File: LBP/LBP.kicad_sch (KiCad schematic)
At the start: 29 parts, among them U1 OPA1641, U2 OPA1641, U3 OPA1641, U4 OPA1641, U5 OPA1641

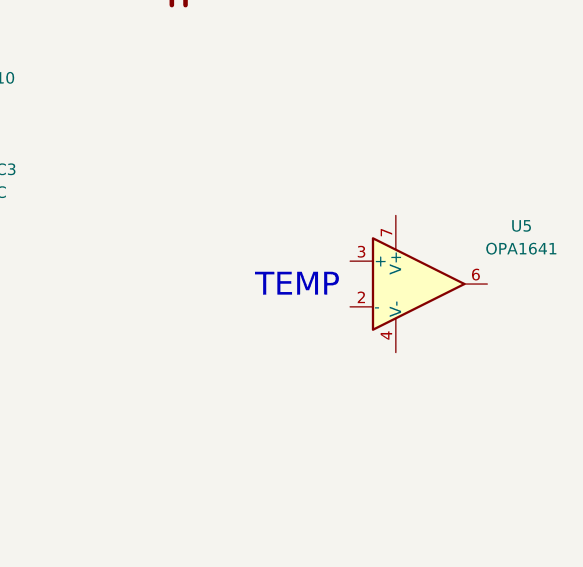
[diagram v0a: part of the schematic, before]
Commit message: LTspice jazz
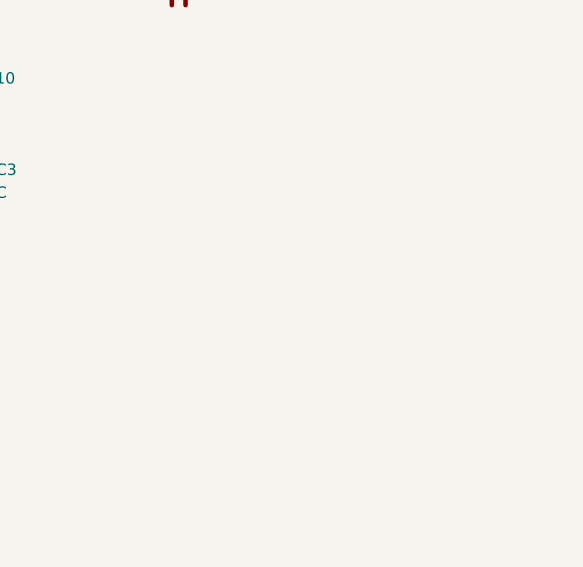
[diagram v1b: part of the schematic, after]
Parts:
- removed U5: OPA1641, symbol Amplifier_Operational:OPA1641
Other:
- note removed: "TEMP"
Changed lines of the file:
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@@
 		(rev "1.0")
-	)
-	(text "TEMP"
-		(exclude_from_sim no)
-		(at 151.638 81.534 0)
-		(effects
-			(font
-				(size 2.54 2.54)
-			)
-		)
 	)
 	(junction
@@
 					(unit 1)
 				)
-			)
-		)
-	)
-	(symbol
-		(lib_id "Amplifier_Operational:OPA1641")
-		(at 165.1 81.28 0)
-		(unit 1)
-		(exclude_from_sim no)
-		(in_bom yes)
-		(on_board yes)
-		(dnp no)
-		(fields_autoplaced yes)
-		(property "Reference" "U5"
-			(at 176.53 74.8598 0)
-			(effects
-				(font
-					(size 1.27 1.27)
-				)
-			)
-		)
-		(property "Value" "OPA1641"
-			(at 176.53 77.3998 0)
-			(effects
-				(font
-					(size 1.27 1.27)
-				)
-			)
-		)
-		(property "Footprint" ""
-			(at 165.1 81.28 0)
-			(effects
-				(font
-					(size 1.27 1.27)
-				)
-				(hide yes)
-			)
-		)
-		(property "Datasheet" "http://www.ti.com/lit/ds/symlink/opa1641.pdf"
-			(at 165.1 81.28 0)
-			(effects
-				(font
-					(size 1.27 1.27)
-				)
-				(hide yes)
-			)
-		)
-		(property "Description" "JFET input, ultralow distortion, low-noise operational amplifier, SOIC-8/VSSOP-8"
-			(at 165.1 81.28 0)
-			(effects
-				(font
-					(size 1.27 1.27)
-				)
-				(hide yes)
-			)
-		)
-		(pin "2"
-		)
-		(pin "3"
-		)
-		(pin "7"
-		)
-		(pin "1"
-		)
-		(pin "5"
-		)
-		(pin "8"
-		)
-		(pin "4"
-		)
-		(pin "6"
-		)
-		(instances
-			(project "LBP"
-				(path "/e9c605b8-0261-4625-b036-2a547cf6d32d"
-					(reference "U5")
-					(unit 1)
-				)
